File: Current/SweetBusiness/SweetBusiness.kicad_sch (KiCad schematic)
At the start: 57 parts, among them J2 I2C, J4 USB, U0 RP2040, U1 MT2492, U2 W25Q128JVS, U3 USBLC6-2SC6, Y0 CSTCE12M0G55-R0

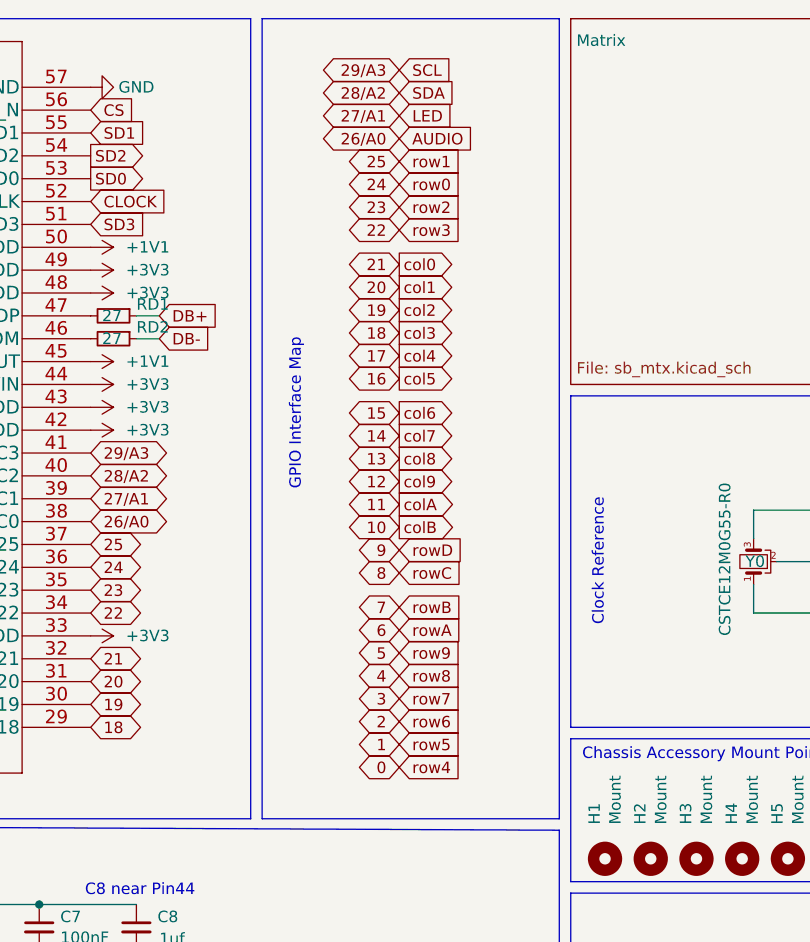
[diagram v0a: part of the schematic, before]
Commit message: Updates to Hardlight, to EDI footprint gallery
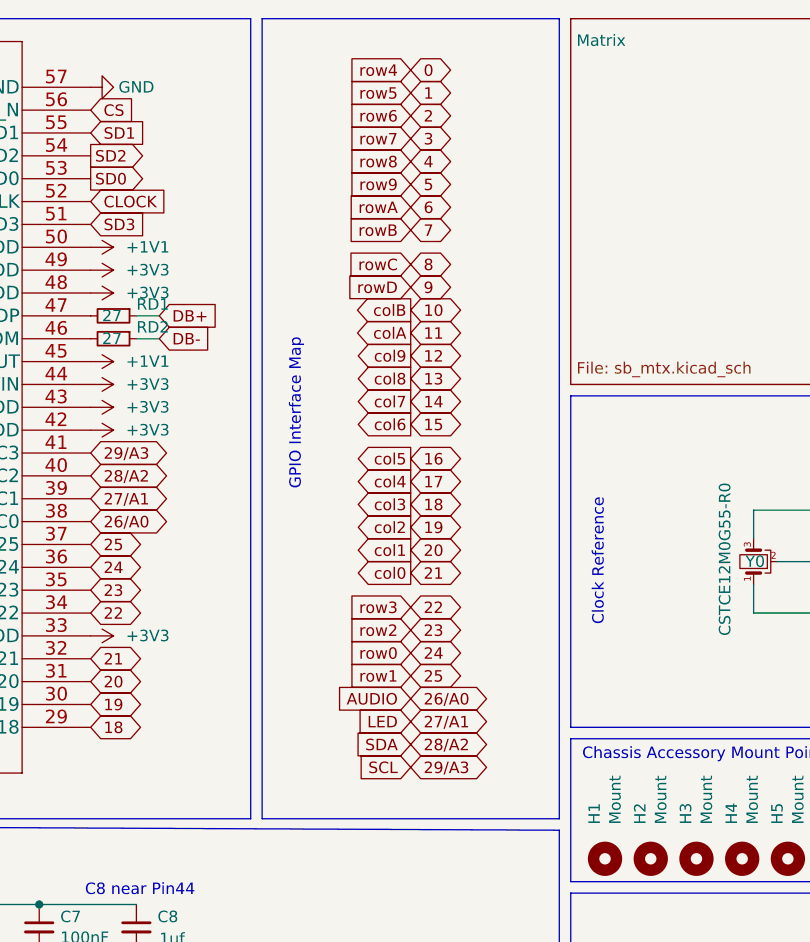
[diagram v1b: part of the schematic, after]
